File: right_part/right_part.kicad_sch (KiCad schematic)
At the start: 46 parts, among them J1 OLED_128x32, SW1 SW_Push_45deg, SW10 SW_Push_45deg, SW11 SW_Push_45deg, SW12 SW_Push_45deg, SW13 SW_Push_45deg, SW14 SW_Push_45deg, SW15 SW_Push_45deg, SW16 SW_Push_45deg, SW17 SW_Push_45deg, SW18 SW_Push_45deg, SW19 SW_Push_45deg, SW2 SW_Push_45deg, SW20 SW_Push_45deg, SW21 SW_Push_45deg, SW3 SW_Push_45deg, SW4 SW_Push_45deg, SW5 SW_Push_45deg, SW6 SW_Push_45deg, SW7 SW_Push_45deg, SW8 SW_Push_45deg, SW9 SW_Push_45deg, U1 Nice_Nano_V2

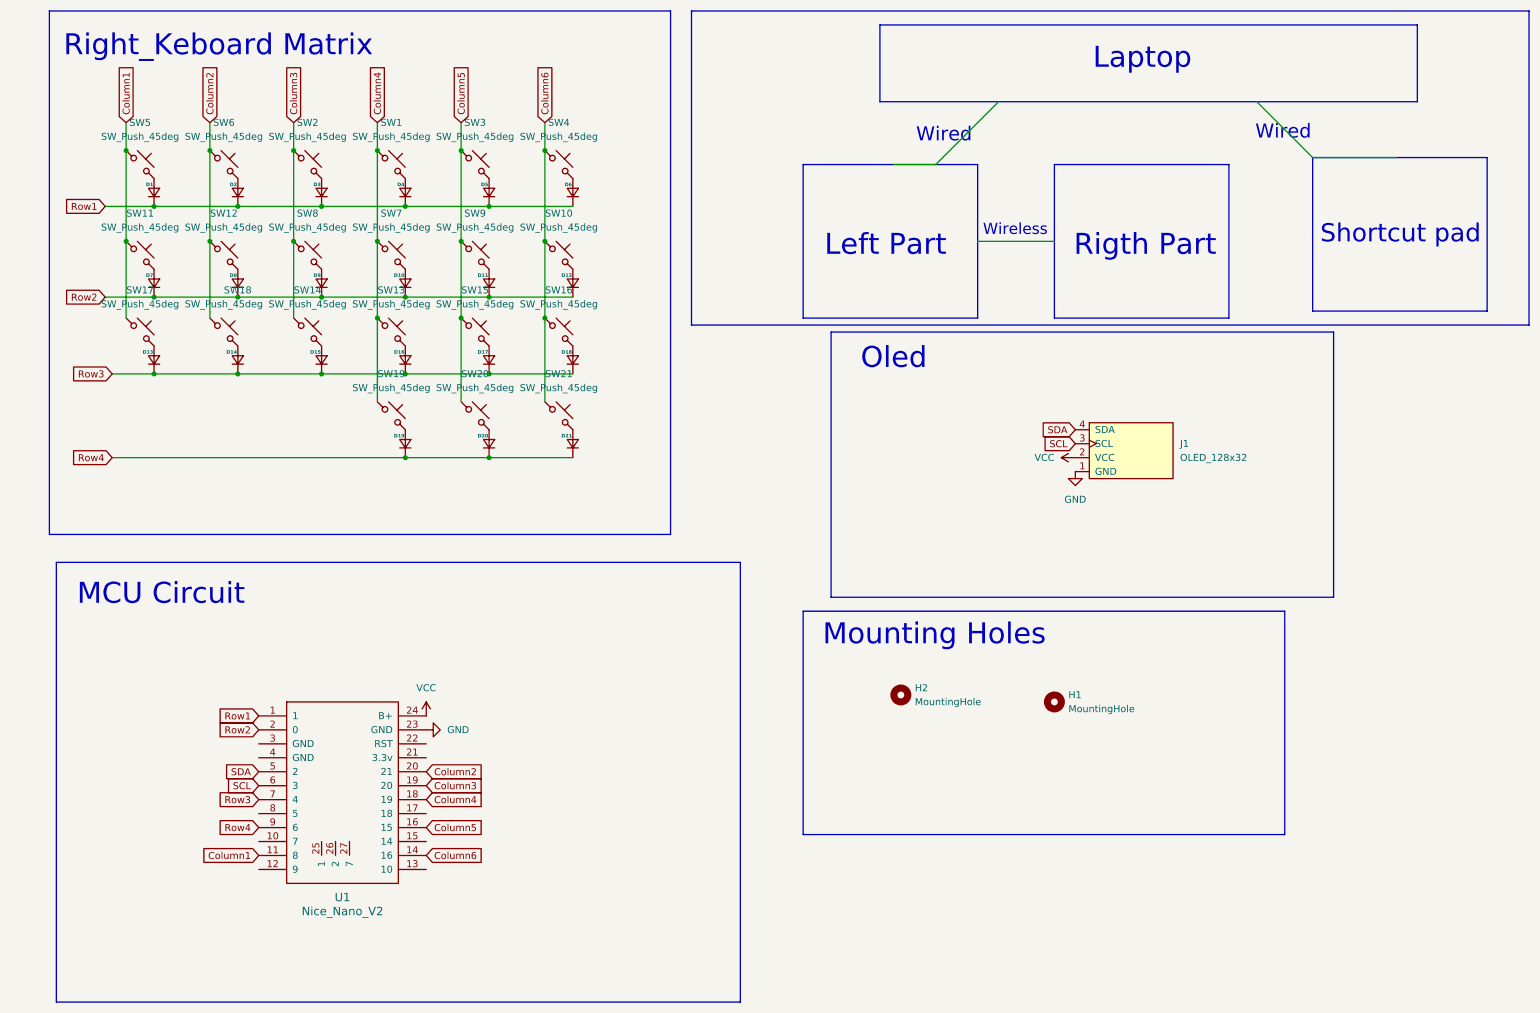
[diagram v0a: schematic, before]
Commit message: right pcb
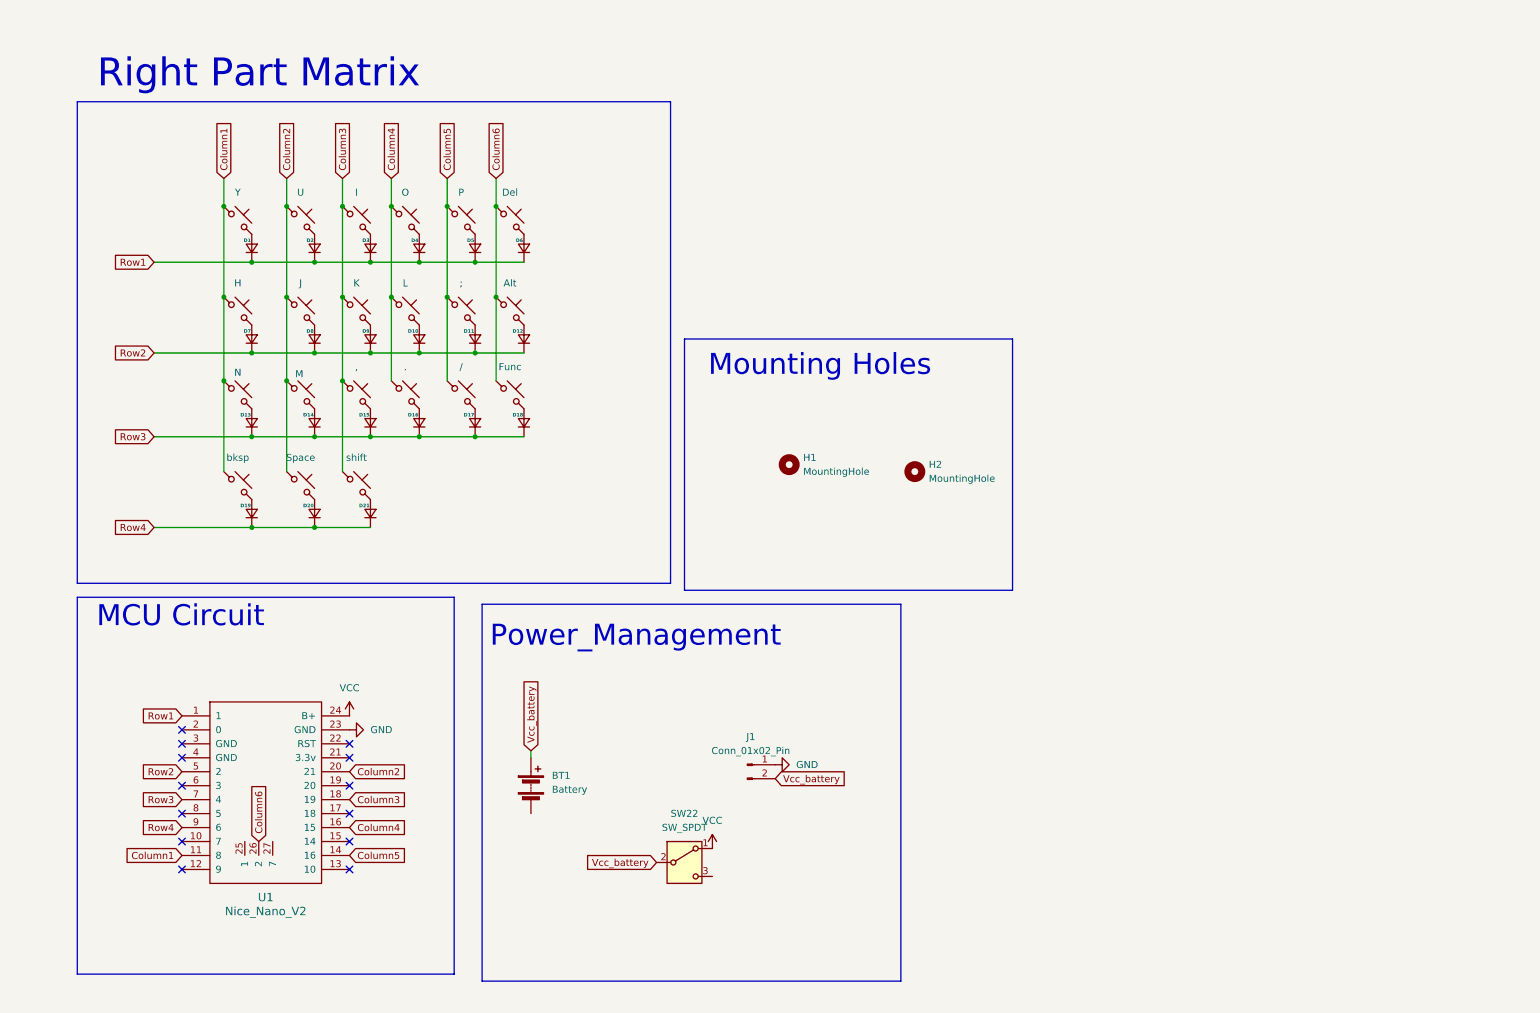
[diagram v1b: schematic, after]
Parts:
- removed J1: OLED_128x32, ScottoKeebs_Components:OLED_128x32, symbol ScottoKeebs:OLED_128x32
- added BT1: Battery, symbol Device:Battery
- added J1: Conn_01x02_Pin, Connector_JST:JST_PH_S2B-PH-K_1x02_P2.00mm_Horizontal, symbol Connector:Conn_01x02_Pin
- added SW22: SW_SPDT, Button_Switch_THT:SW_Slide_SPDT_Angled_CK_OS102011MA1Q, symbol Switch:SW_SPDT
- SW1: value SW_Push_45deg -> I
- SW10: value SW_Push_45deg -> H
- SW11: value SW_Push_45deg -> ;
- SW12: value SW_Push_45deg -> Alt
- SW13: value SW_Push_45deg -> ,
- SW14: value SW_Push_45deg -> M
- SW15: value SW_Push_45deg -> .
- SW16: value SW_Push_45deg -> N
- SW17: value SW_Push_45deg -> /
- SW18: value SW_Push_45deg -> Func
- SW19: value SW_Push_45deg -> shift
- SW2: value SW_Push_45deg -> U
- SW20: value SW_Push_45deg -> bksp; footprint ScottoKeebs_MX:MX_PCB_1.00u -> ScottoKeebs_MX:MX_PCB_1.50u
- SW21: value SW_Push_45deg -> Space; footprint ScottoKeebs_MX:MX_PCB_1.50u -> ScottoKeebs_MX:MX_PCB_1.00u
- SW3: value SW_Push_45deg -> O
- SW4: value SW_Push_45deg -> Y
- SW5: value SW_Push_45deg -> P
- SW6: value SW_Push_45deg -> Del
- SW7: value SW_Push_45deg -> K
- SW8: value SW_Push_45deg -> J
- SW9: value SW_Push_45deg -> L
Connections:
- net SDA is gone; now on net Row2: U1.5 (2)
- net Column1: now also SW10.1, SW16.1, SW20.1, SW4.1; no longer SW11.1, SW17.1, SW5.1
- net Column2: now also SW14.1, SW2.1, SW21.1, SW8.1; no longer SW12.1, SW18.1, SW6.1
- net Column3: now also SW1.1, SW13.1, SW19.1, SW7.1, U1.18 (19); no longer SW14.1, SW2.1, SW8.1, U1.19 (20)
- net Column4: now also SW15.1, SW3.1, SW9.1, U1.16 (15); no longer SW1.1, SW13.1, SW19.1, SW7.1, U1.18 (19)
- net Column5: now also SW11.1, SW17.1, SW5.1, U1.14 (16); no longer SW15.1, SW20.1, SW3.1, SW9.1, U1.16 (15)
- net Column6: now also SW12.1, SW18.1, SW6.1, U1.26 (2); no longer SW10.1, SW16.1, SW21.1, SW4.1, U1.14 (16)
- net GND: now also J1.1 (Pin_1)
- net Row2: no longer U1.2 (0)
- net VCC: now also SW22.1 (A)
- net at D18.2 (A): now also SW18.2; no longer SW16.2
- net at SW20.2: now also D19.2 (A); no longer D20.2 (A)
- net at SW7.2: now also D9.2 (A); no longer D10.2 (A)
- net at D11.2 (A): now also SW11.2; no longer SW9.2
- net at SW19.2: now also D21.2 (A); no longer D19.2 (A)
- net at D6.2 (A): now also SW6.2; no longer SW4.2
- net at SW2.2: now also D2.2 (A); no longer D3.2 (A)
- net at SW10.2: now also D7.2 (A); no longer D12.2 (A)
- net at D15.2 (A): now also SW13.2; no longer SW14.2
- net at D5.2 (A): now also SW5.2; no longer SW3.2
- net at SW21.2: now also D20.2 (A); no longer D21.2 (A)
- net at D16.2 (A): now also SW15.2; no longer SW13.2
- net at D1.2 (A): now also SW4.2; no longer SW5.2
- net at SW8.2: now also D8.2 (A); no longer D9.2 (A)
- net at D17.2 (A): now also SW17.2; no longer SW15.2
- net at SW1.2: now also D3.2 (A); no longer D4.2 (A)
- net at D13.2 (A): now also SW16.2; no longer SW17.2
- net at SW12.2: now also D12.2 (A); no longer D8.2 (A)
- net at D14.2 (A): now also SW14.2; no longer SW18.2
- net SCL: no longer names the net of U1.6 (3)
- new net: D10.2 (A), SW9.2
- new net: D4.2 (A), SW3.2
- new net Vcc_battery: BT1.1 (+), J1.2 (Pin_2), SW22.2 (B)
- no-connect marks 0 -> 13
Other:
- note added: "Power_Management"
- note added: "Right Part Matrix"
- note removed: "Laptop"
- note removed: "Left Part"
- note removed: "Oled"
- note removed: "Right_Keboard Matrix"
- note removed: "Rigth Part"
- note removed: "Shortcut pad"
- note removed: "Wired"
- note removed: "Wireless"
- title: Left_Part -> (none)
